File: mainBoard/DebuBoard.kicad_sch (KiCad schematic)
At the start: 9 parts, among them J1 Conn_01x04, J31 Conn_02x05_Odd_Even, J7 Conn_01x05

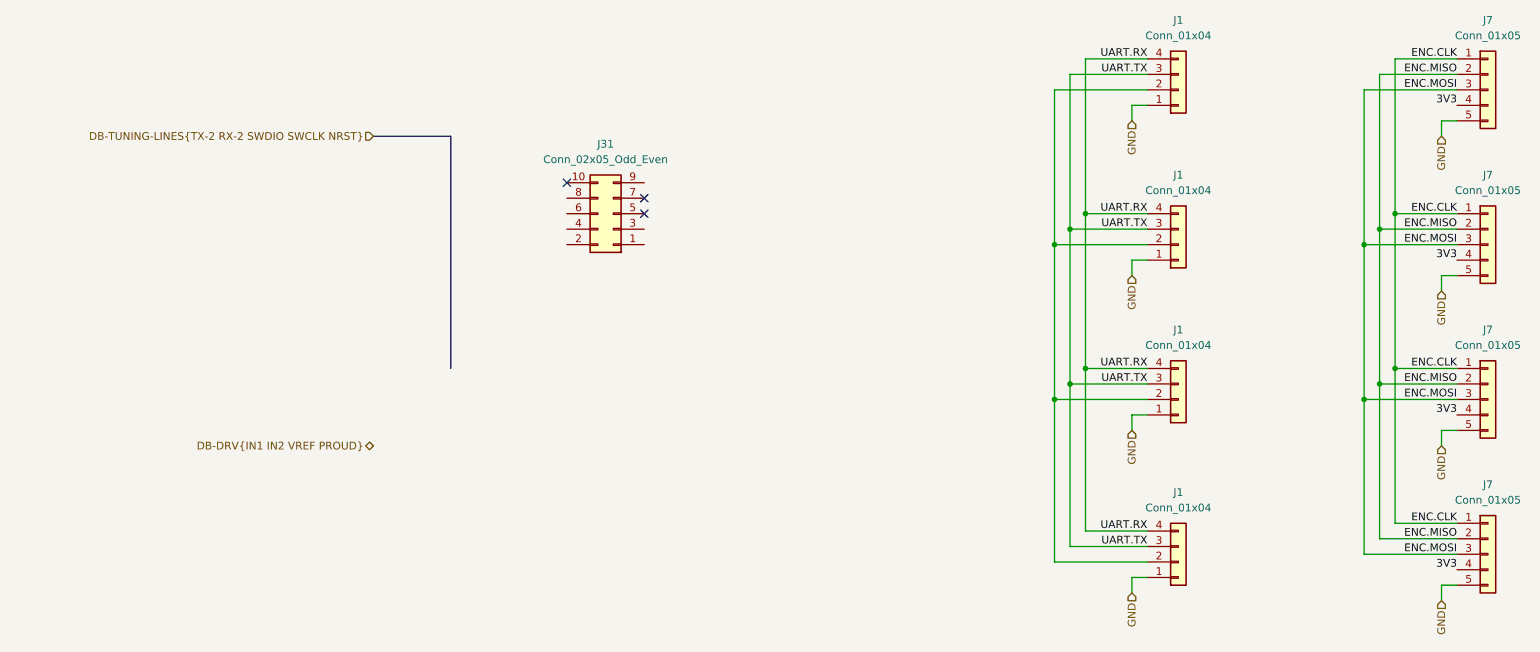
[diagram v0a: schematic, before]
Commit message: ukild
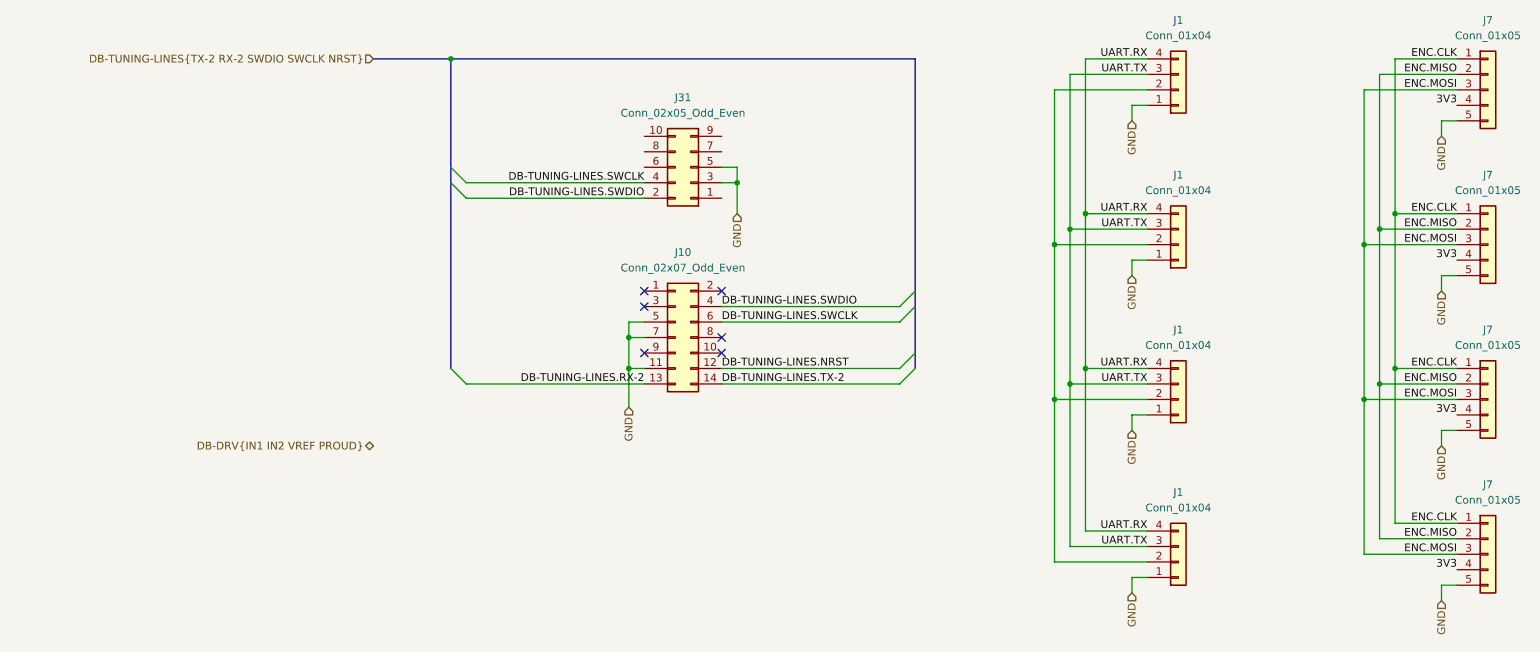
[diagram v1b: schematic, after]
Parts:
- added J10: Conn_02x07_Odd_Even, Connector_PinHeader_1.27mm:PinHeader_2x07_P1.27mm_Vertical_SMD, symbol Connector_Generic:Conn_02x07_Odd_Even
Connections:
- net GND: now also J31.3 (Pin_3), J31.5 (Pin_5), J10.11 (Pin_11), J10.5 (Pin_5), J10.7 (Pin_7)
- net DB-TUNING-LINES.SWDIO: now reaches J31.2 (Pin_2)
- net DB-TUNING-LINES.SWDIO: now also J10.4 (Pin_4)
- net DB-TUNING-LINES.SWCLK: now reaches J31.4 (Pin_4)
- net DB-TUNING-LINES.SWCLK: now also J10.6 (Pin_6)
- new net DB-TUNING-LINES.NRST: J10.12 (Pin_12)
- new net DB-TUNING-LINES.RX-2: J10.13 (Pin_13)
- new net DB-TUNING-LINES.TX-2: J10.14 (Pin_14)
- no-connect marks 3 -> 6
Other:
- moved on the sheet: J31
